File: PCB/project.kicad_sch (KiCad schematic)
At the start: 31 parts, among them J4 Conn_01x10, K1 Компрессор, K2 ТЕН поддон, K3 ТЕН компрессор, Q1 IRLML0030, Q2 IRLML0030, Q3 IRLML0030, U1 STM32F030F4Px, U2 EL814, U3 EL814

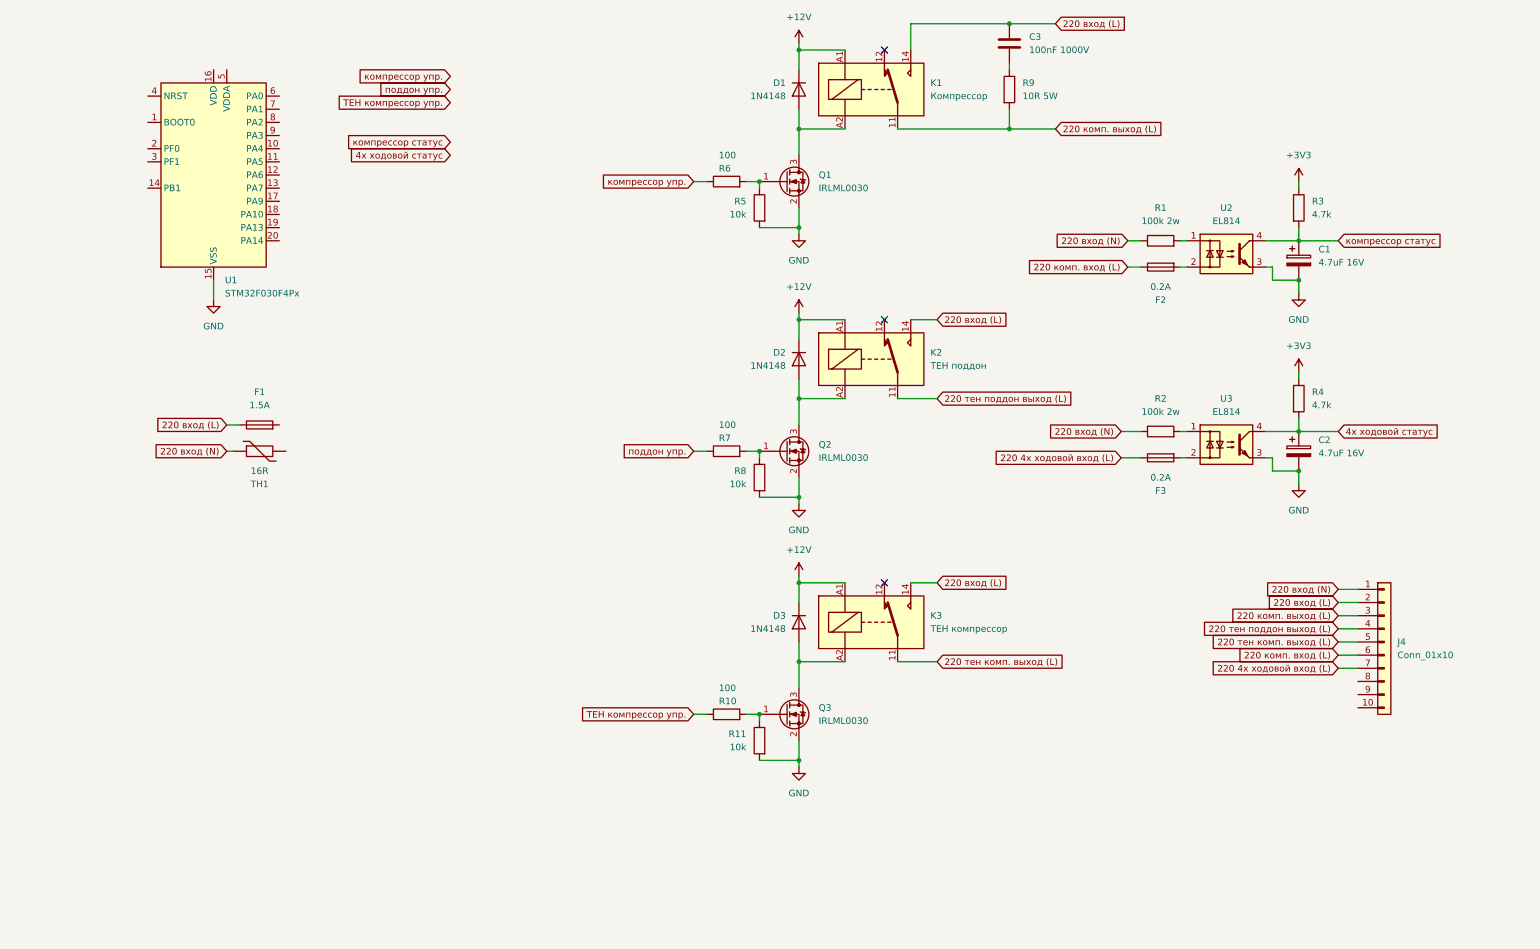
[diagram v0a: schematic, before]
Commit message: Updated schematic(not finished)
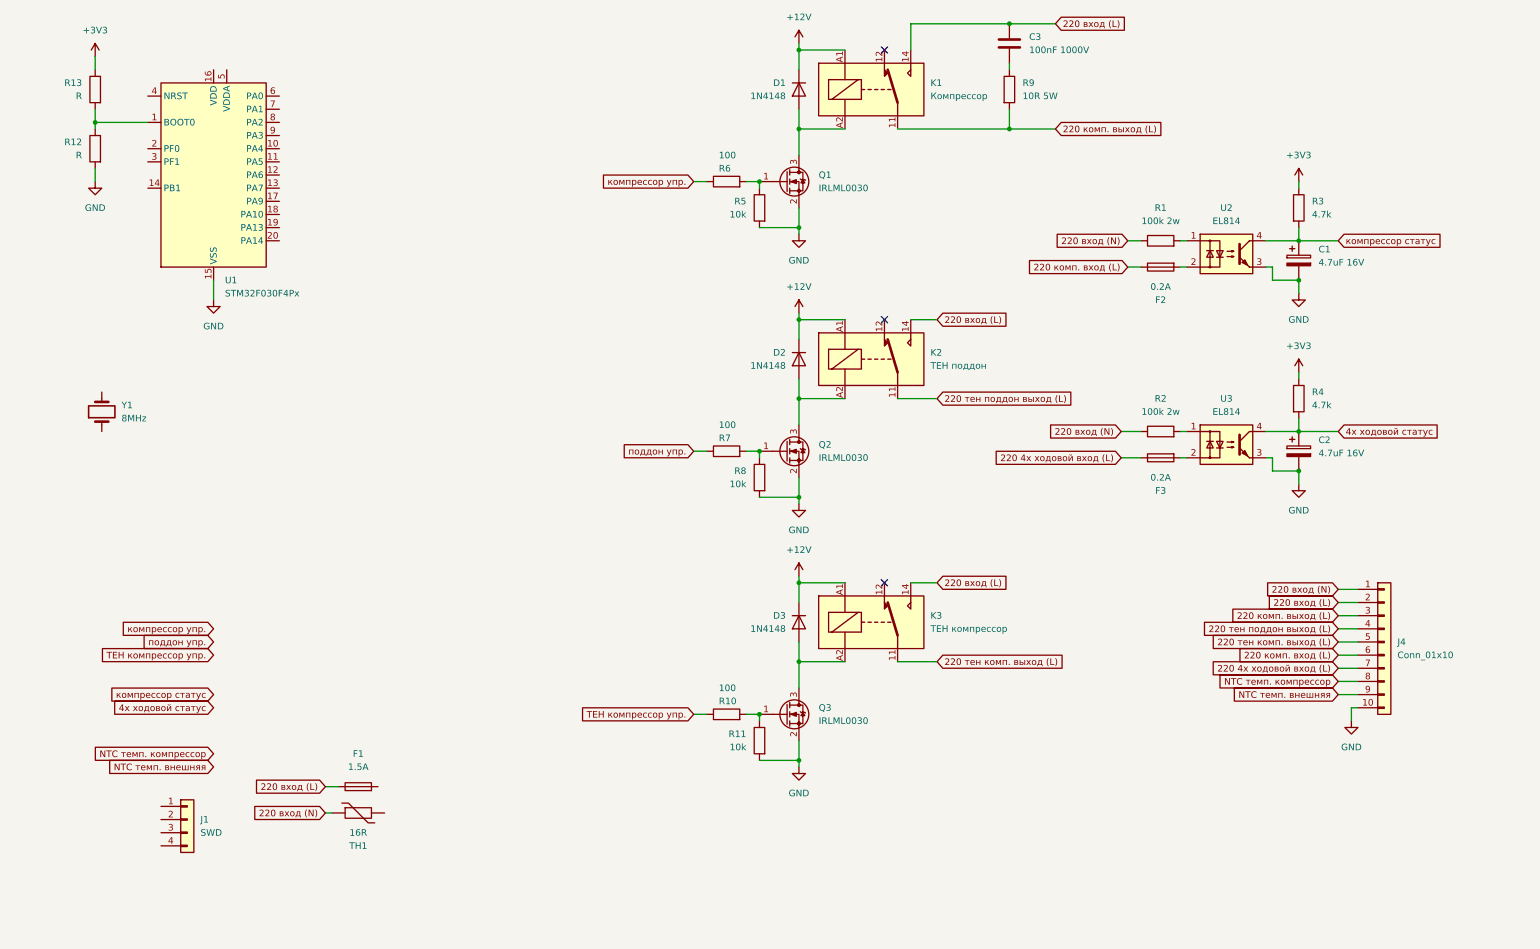
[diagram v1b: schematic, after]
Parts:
- added J1: SWD, Connector_PinHeader_2.54mm:PinHeader_1x04_P2.54mm_Vertical, symbol Connector_Generic:Conn_01x04
- added R12, R13: R, Resistor_SMD:R_0805_2012Metric_Pad1.20x1.40mm_HandSolder, symbol Device:R
- added Y1: 8MHz, Crystal:Crystal_HC18-U_Vertical, symbol Device:Crystal
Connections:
- net +3V3: now also R13.1
- net GND: now also J4.10 (Pin_10), R12.2
- net at U1.1 (BOOT0): now also R12.1, R13.2
- net NTC темп. компрессор: now reaches J4.8 (Pin_8)
- net NTC темп. внешняя: now reaches J4.9 (Pin_9)
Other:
- moved on the sheet: F1, TH1

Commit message: Updated PCB (still not finished)
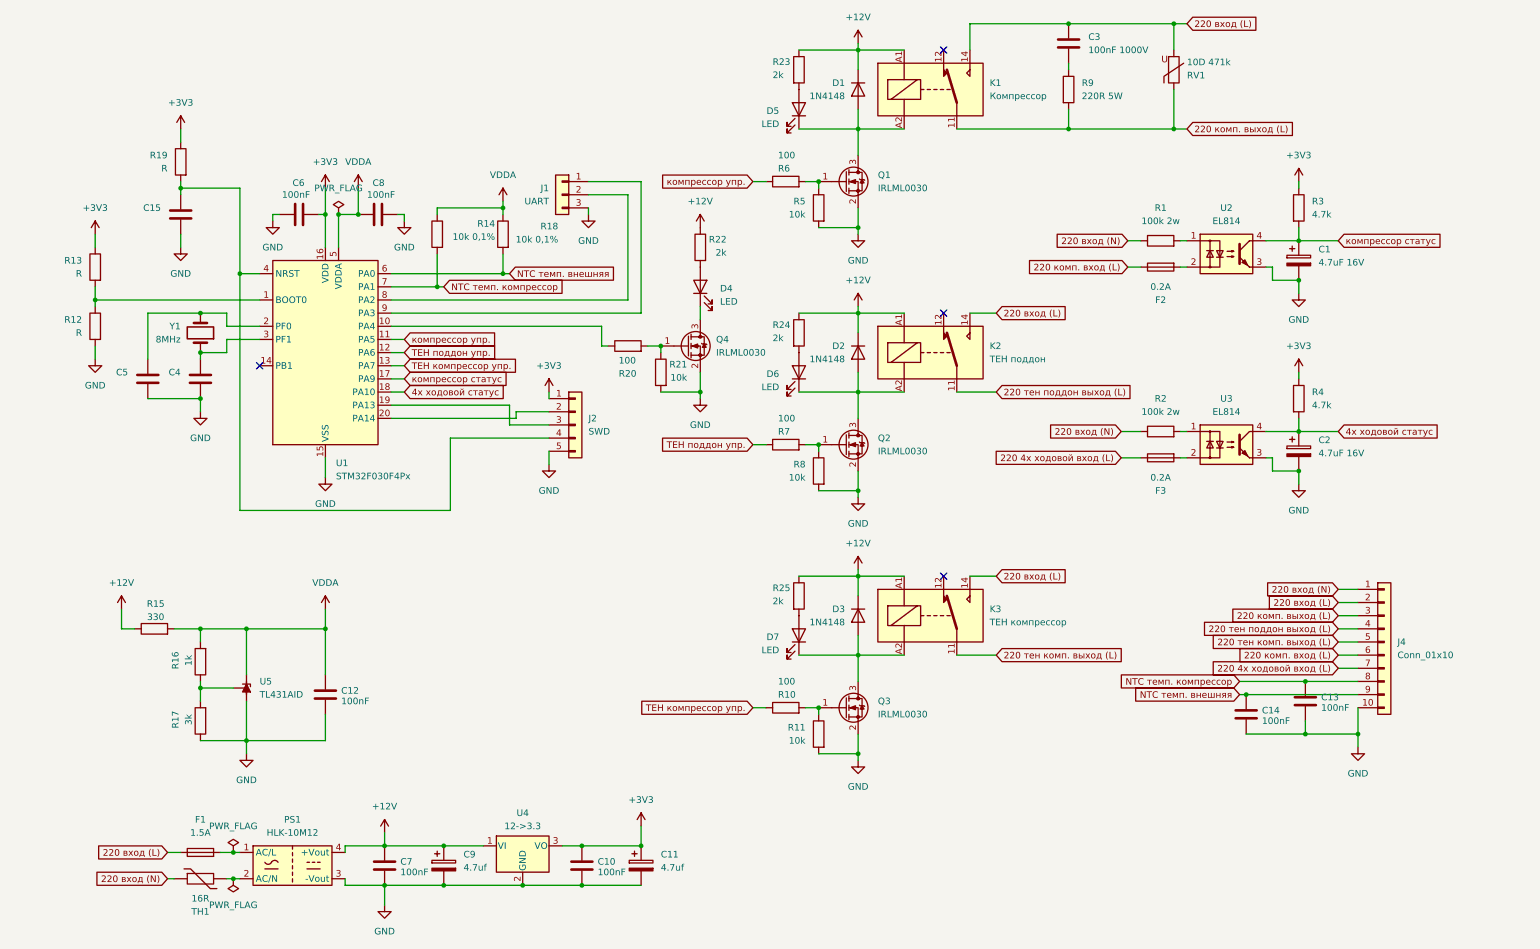
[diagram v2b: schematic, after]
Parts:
- removed J1: SWD, Connector_PinHeader_2.54mm:PinHeader_1x04_P2.54mm_Vertical, symbol Connector_Generic:Conn_01x04
- added C10, C12, C13, C14, C6, C7, C8: 100nF, Capacitor_SMD:C_0805_2012Metric_Pad1.18x1.45mm_HandSolder, symbol Device:C
- added C11, C9: 4.7uf, Capacitor_THT:CP_Radial_D5.0mm_P2.50mm, symbol Device:C_Polarized
- added C15, C4, C5: C, Capacitor_SMD:C_0805_2012Metric_Pad1.18x1.45mm_HandSolder, symbol Device:C
- added D4, D5, D6, D7: LED, LED_THT:LED_D3.0mm, symbol Device:LED
- added J1: UART, Connector_PinHeader_2.54mm:PinHeader_1x03_P2.54mm_Vertical, symbol Connector_Generic:Conn_01x03
- added J2: SWD, Connector_PinHeader_2.54mm:PinHeader_1x05_P2.54mm_Vertical, symbol Connector_Generic:Conn_01x05
- added PS1: HLK-10M12, Converter_ACDC:Converter_ACDC_Hi-Link_HLK-10Mxx, symbol Converter_ACDC:HLK-10M12
- added Q4: IRLML0030, Package_TO_SOT_SMD:SOT-23W_Handsoldering, symbol Transistor_FET:IRLML0030
- added R14, R18: 10k 0,1%, Resistor_SMD:R_1206_3216Metric_Pad1.30x1.75mm_HandSolder, symbol Device:R
- added R15: 330, Resistor_SMD:R_1206_3216Metric_Pad1.30x1.75mm_HandSolder, symbol Device:R
- added R16: 1k, Resistor_SMD:R_1206_3216Metric_Pad1.30x1.75mm_HandSolder, symbol Device:R
- added R17: 3k, Resistor_SMD:R_1206_3216Metric_Pad1.30x1.75mm_HandSolder, symbol Device:R
- added R19: R, Resistor_SMD:R_0805_2012Metric_Pad1.20x1.40mm_HandSolder, symbol Device:R
- added R20: 100, Resistor_SMD:R_0805_2012Metric_Pad1.20x1.40mm_HandSolder, symbol Device:R
- added R21: 10k, Resistor_SMD:R_0805_2012Metric_Pad1.20x1.40mm_HandSolder, symbol Device:R
- added R22, R23, R24, R25: 2k, Resistor_SMD:R_0805_2012Metric_Pad1.20x1.40mm_HandSolder, symbol Device:R
- added RV1: 10D 471k, Varistor:RV_Disc_D9mm_W3.4mm_P5mm, symbol Device:Varistor
- added U4: 12->3.3, Package_TO_SOT_THT:TO-220-3_Vertical, symbol Regulator_Linear:LM7805_TO220
- added U5: TL431AID, Package_TO_SOT_SMD:SOT-23_Handsoldering, symbol Reference_Voltage:TL431DBZ
- R9: value 10R 5W -> 220R 5W
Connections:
- net поддон упр. is gone; now on net ТЕН поддон упр.: R7.1
- net +12V: now also C7.1, C9.1, PS1.4 (+Vout), R15.1, R22.1, R23.1, R24.1, R25.1, U4.1 (VI)
- net +3V3: now also U1.16 (VDD), C10.1, C11.1, C6.1, J2.1 (Pin_1), R19.1, U4.3 (VO)
- net 220 вход (L): now also RV1.2
- net 220 комп. выход (L): now also RV1.1
- net 4х ходовой статус: now also U1.18 (PA10)
- net GND: now also C10.2, C11.2, C12.2, C13.2, C14.2, C15.2, C4.2, C5.2, C6.2, C7.2, C8.2, C9.2, J1.3 (Pin_3), J2.5 (Pin_5), PS1.3 (-Vout), Q4.2 (S), R17.1, R21.2, U4.2 (GND), U5.3 (A)
- net NTC темп. внешняя: now also U1.6 (PA0), C14.1, R18.2
- net NTC темп. компрессор: now also U1.7 (PA1), C13.1, R14.2
- net ТЕН компрессор упр.: now also U1.13 (PA7)
- net компрессор статус: now also U1.17 (PA9)
- net компрессор упр.: now also U1.11 (PA5)
- net at D1.2 (A), K1.A2, Q1.3 (D): now also D5.1 (K)
- net at U1.10 (PA4): now also R20.1
- net ТЕН поддон упр.: now reaches U1.12 (PA6)
- net at U1.19 (PA13): now also J2.3 (Pin_3)
- net at U1.2 (PF0): now also Y1.2, C5.1
- net at U1.20 (PA14): now also J2.2 (Pin_2)
- net at U1.3 (PF1): now also Y1.1, C4.1
- net at U1.4 (NRST): now also C15.1, J2.4 (Pin_4), R19.2
- net VDDA: now reaches U1.5 (VDDA)
- net VDDA: now also C12.1, C8.1, R14.1, R15.2, R16.2, R18.1, U5.1 (K)
- net at U1.8 (PA2): now also J1.2 (Pin_2)
- net at U1.9 (PA3): now also J1.1 (Pin_1)
- net at D3.2 (A), K3.A2, Q3.3 (D): now also D7.1 (K)
- net at TH1.2: now also PS1.2 (AC/N)
- net at D2.2 (A), K2.A2, Q2.3 (D): now also D6.1 (K)
- net at F1.2: now also PS1.1 (AC/L)
- new net: Q4.1 (G), R20.2, R21.1
- new net: D5.2 (A), R23.2
- new net: R16.1, R17.2, U5.2 (REF)
- new net: D4.1 (K), Q4.3 (D)
- new net: D4.2 (A), R22.2
- new net: D7.2 (A), R25.2
- new net: D6.2 (A), R24.2
- no-connect marks 3 -> 4
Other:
- moved on the sheet: C3, D1, D2, D3, F1, K1, K2, K3, Q1, Q2, Q3, R10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

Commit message: PCB and schematic done
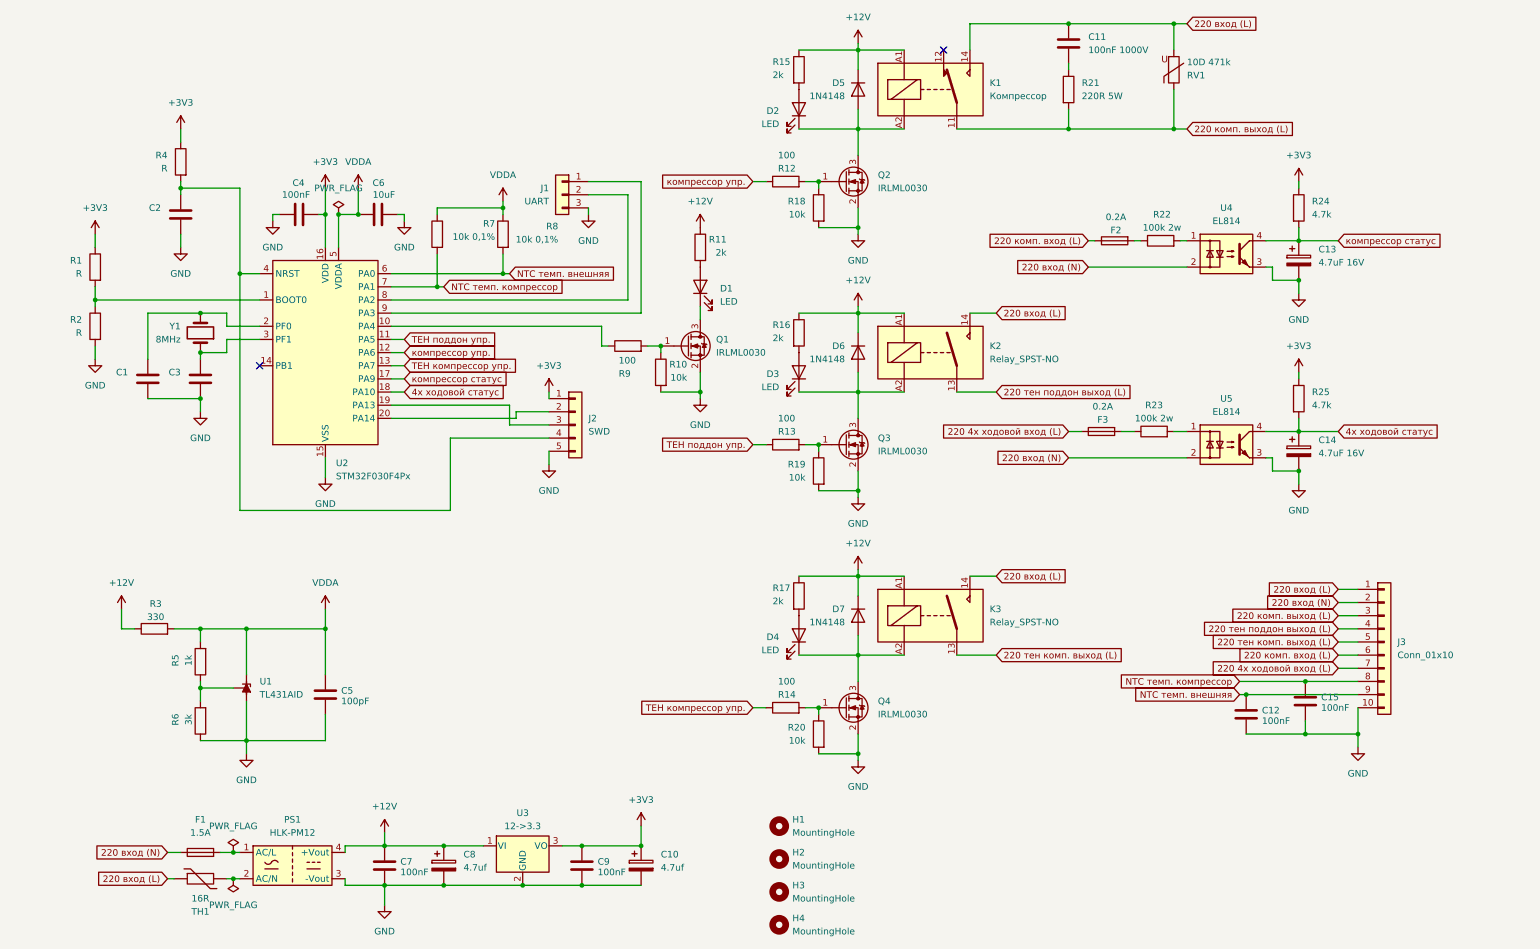
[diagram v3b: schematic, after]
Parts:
- removed K2: ТЕН поддон, Relay_THT:Relay_SPDT_Hongfa_HF3F-L-xx-1ZL1T, symbol Relay:Relay_SPDT
- removed K3: ТЕН компрессор, Relay_THT:Relay_SPDT_Hongfa_HF3F-L-xx-1ZL1T, symbol Relay:Relay_SPDT
- removed PS1: HLK-10M12, Converter_ACDC:Converter_ACDC_Hi-Link_HLK-10Mxx, symbol Converter_ACDC:HLK-10M12
- added H1, H2, H3, H4: MountingHole, MountingHole:MountingHole_3.2mm_M3, symbol Mechanical:MountingHole
- added K2, K3: Relay_SPST-NO, Relay_THT:Relay_SPST_Schrack-RP-II-1-FormA_RM3.5mm, symbol Relay:Relay_SPST-NO
- added PS1: HLK-PM12, Converter_ACDC:Converter_ACDC_Hi-Link_HLK-PMxx, symbol Converter_ACDC:HLK-PM12
- C5: renamed from C12; value 100nF -> 100pF
- C6: renamed from C8; value 100nF -> 10uF
- J3: renamed from J4; footprint Connector_Phoenix_MSTB:PhoenixContact_MSTBA_2,5_10-G_1x10_P5.00mm_Horizontal -> Connector_Phoenix_MSTB:PhoenixContact_MSTB_2,5_10-GF-5,08_1x10_P5.08mm_Horizontal_ThreadedFlange
- renumbered C5 to C1, C11 to C10, C3 to C11, C14 to C12, C1 to C13, C2 to C14, C13 to C15, C15 to C2, C4 to C3, C6 to C4, C9 to C8, C10 to C9, D4 to D1, D5 to D2, D6 to D3, D7 to D4, D1 to D5, D2 to D6, D3 to D7, Q4 to Q1, Q1 to Q2, Q2 to Q3, Q3 to Q4, R13 to R1, R21 to R10, R22 to R11, R6 to R12, R7 to R13, R10 to R14, R23 to R15, R24 to R16, R25 to R17, R5 to R18, R8 to R19, R12 to R2, R11 to R20, R9 to R21, R1 to R22, R2 to R23, R3 to R24, R4 to R25, R15 to R3, R19 to R4, R16 to R5, R17 to R6, R14 to R7, R18 to R8, R20 to R9, U5 to U1, U1 to U2, U4 to U3, U2 to U4, U3 to U5
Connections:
- net +12V: now also K2.A1, K3.A1, PS1.4 (+Vout)
- net 220 вход (L): now also J3.1 (Pin_1), TH1.1, K2.14, K3.14; no longer F1.1, J3.2 (Pin_2)
- net 220 вход (N): now also F1.1, J3.2 (Pin_2), U4.2, U5.2; no longer J3.1 (Pin_1), R22.1, R23.1, TH1.1
- net 220 тен комп. выход (L): now also K3.13
- net 220 тен поддон выход (L): now also K2.13
- net GND: now also PS1.3 (-Vout)
- net ТЕН поддон упр.: now also U2.11 (PA5); no longer U2.12 (PA6)
- net компрессор упр.: now also U2.12 (PA6); no longer U2.11 (PA5)
- net at F2.2: now also R22.1; no longer U4.2
- net at D4.1 (K), D7.2 (A), Q4.3 (D): now also K3.A2
- net at F3.2: now also R23.1; no longer U5.2
- net at F1.2: now also PS1.1 (AC/L)
- net at TH1.2: now also PS1.2 (AC/N)
- net at D3.1 (K), D6.2 (A), Q3.3 (D): now also K2.A2
- no-connect marks 4 -> 2
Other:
- moved on the sheet: F2, F3, R23
